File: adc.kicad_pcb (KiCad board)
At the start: 2 copper layers, 53.8 x 69.1 mm, 88 parts, among them J1 Conn_02x08_Odd_Even, J2 Conn_02x08_Odd_Even, J3 Conn_02x08_Odd_Even, J4 Conn_02x08_Odd_Even, J5 Conn_01x04_Male, J9 Conn_02x08_Odd_Even, U1 ADC128D818, U2 ADC128D818, U3 ADC128D818, U4 ADC128D818, U5 ADC128D818

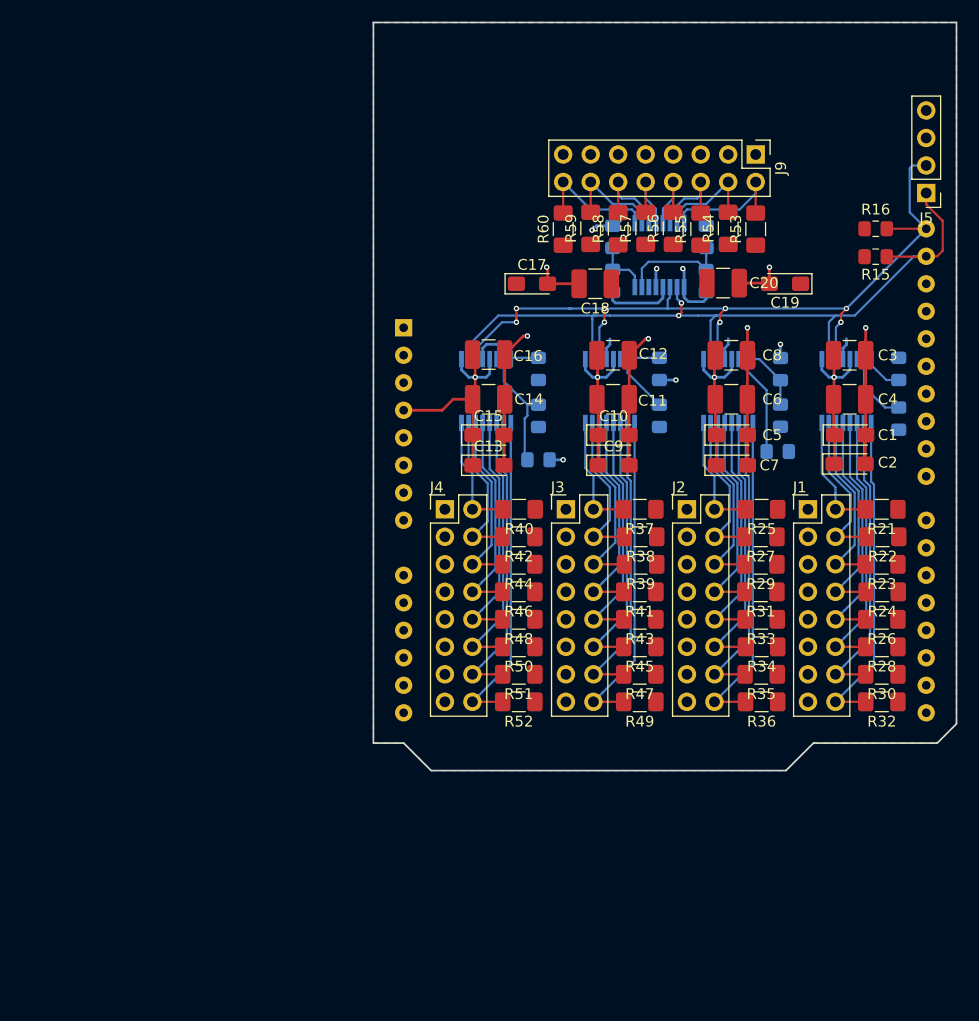
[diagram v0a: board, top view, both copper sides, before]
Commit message: silkscreen
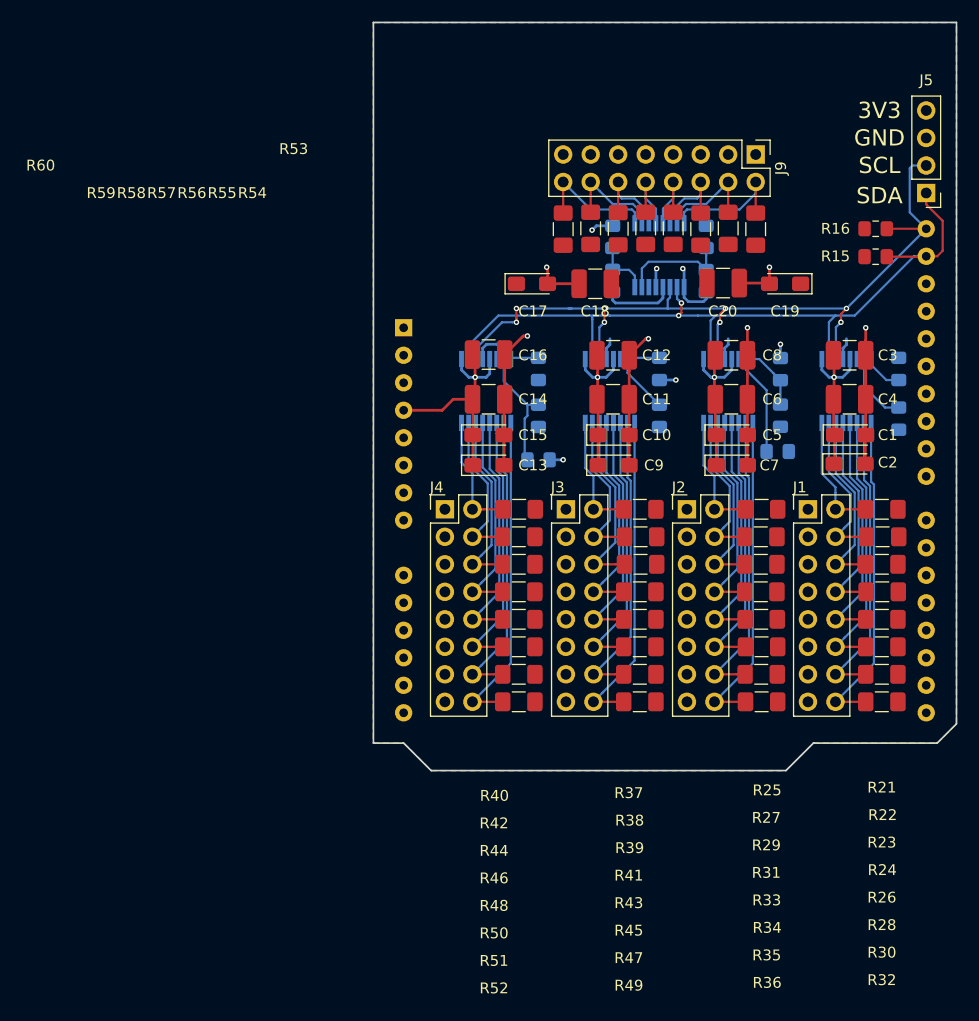
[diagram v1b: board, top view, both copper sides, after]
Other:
- board text added: "3V3"
- board text added: "GND"
- board text added: "SCL"
- board text added: "SDA"
